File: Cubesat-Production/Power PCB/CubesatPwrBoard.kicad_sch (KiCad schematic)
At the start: 20 parts, among them J1 Conn_01x04_Female, J2 Conn_01x04_Female, J3 Conn_01x04_Female, J5 Conn_01x04_Female, J6 Conn_01x03_Female, J7 Conn_01x03_Female, J8 Conn_01x03_Female

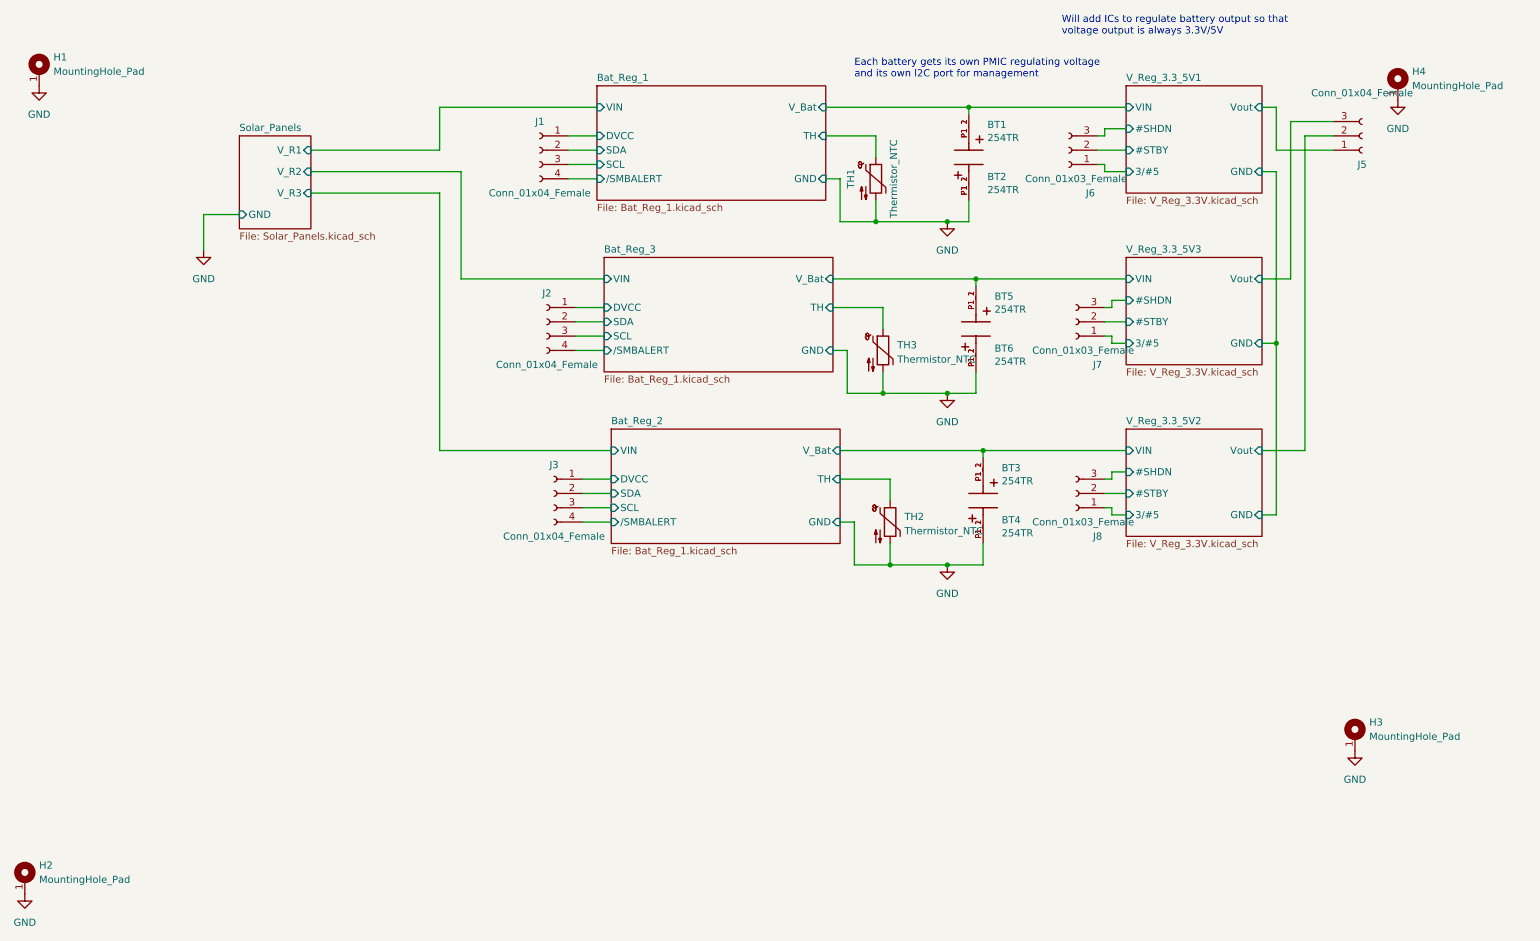
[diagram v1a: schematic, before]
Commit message: Small changes to board before moving to previous-revision
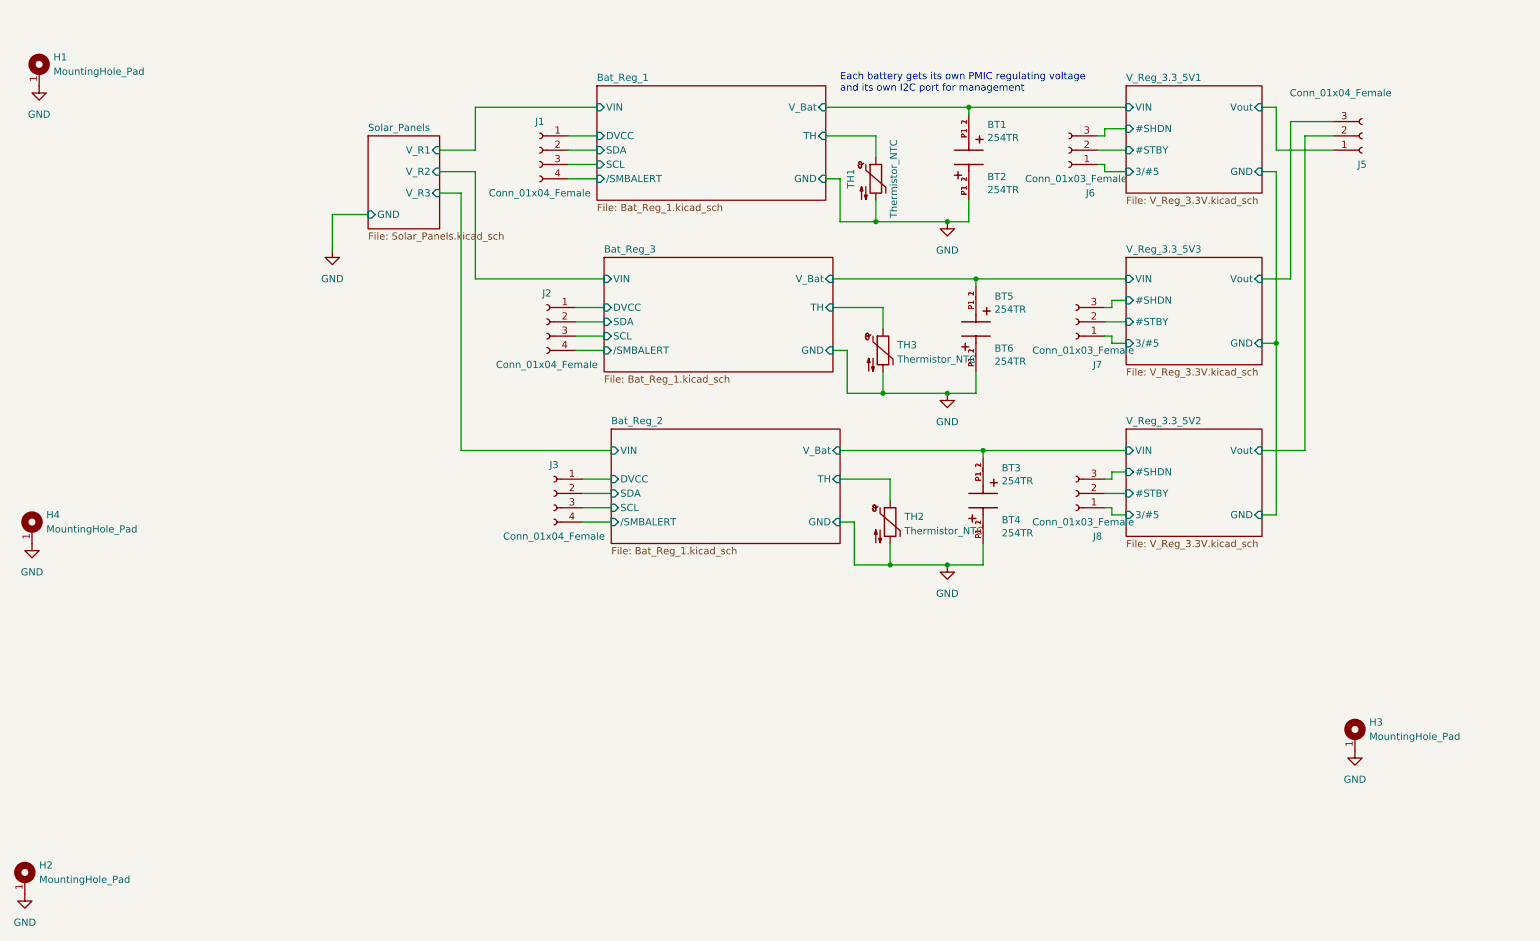
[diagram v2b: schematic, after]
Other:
- note removed: "Will add ICs to regulate battery output so that voltage output is always 3.3V/5V"
- moved on the sheet: H4
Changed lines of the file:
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@@
     (stroke (width 0) (type default) (color 0 0 0 0))
   )
-  (wire (pts (xy 60.96 55.88) (xy 67.31 55.88))
+  (wire (pts (xy 83.82 55.88) (xy 90.17 55.88))
     (stroke (width 0) (type default) (color 0 0 0 0))
   )
@@
     (stroke (width 0) (type default) (color 0 0 0 0))
   )
-  (wire (pts (xy 106.68 67.31) (xy 106.68 48.26))
+  (wire (pts (xy 109.22 67.31) (xy 109.22 48.26))
     (stroke (width 0) (type default) (color 0 0 0 0))
   )
@@
     (stroke (width 0) (type default) (color 0 0 0 0))
   )
-  (wire (pts (xy 80.01 44.45) (xy 102.87 44.45))
-    (stroke (width 0) (type default) (color 0 0 0 0))
-  )
   (wire (pts (xy 220.98 105.41) (xy 224.79 105.41))
     (stroke (width 0) (type default) (color 0 0 0 0))
   )
-  (wire (pts (xy 102.87 52.07) (xy 102.87 97.79))
+  (wire (pts (xy 106.68 52.07) (xy 106.68 97.79))
     (stroke (width 0) (type default) (color 0 0 0 0))
   )
@@
     (stroke (width 0) (type default) (color 0 0 0 0))
   )
-  (wire (pts (xy 102.87 97.79) (xy 133.35 97.79))
-    (stroke (width 0) (type default) (color 0 0 0 0))
-  )
   (wire (pts (xy 171.45 41.91) (xy 180.34 41.91))
     (stroke (width 0) (type default) (color 0 0 0 0))
@@
     (stroke (width 0) (type default) (color 0 0 0 0))
   )
+  (wire (pts (xy 102.87 52.07) (xy 106.68 52.07))
+    (stroke (width 0) (type default) (color 0 0 0 0))
+  )
   (wire (pts (xy 193.04 87.63) (xy 198.12 87.63))
     (stroke (width 0) (type default) (color 0 0 0 0))
@@
     (stroke (width 0) (type default) (color 0 0 0 0))
   )
-  (wire (pts (xy 60.96 62.23) (xy 60.96 55.88))
+  (wire (pts (xy 83.82 62.23) (xy 83.82 55.88))
+    (stroke (width 0) (type default) (color 0 0 0 0))
+  )
+  (wire (pts (xy 109.22 36.83) (xy 130.81 36.83))
     (stroke (width 0) (type default) (color 0 0 0 0))
   )
@@
     (stroke (width 0) (type default) (color 0 0 0 0))
   )
+  (wire (pts (xy 102.87 48.26) (xy 109.22 48.26))
+    (stroke (width 0) (type default) (color 0 0 0 0))
+  )
   (wire (pts (xy 222.25 109.22) (xy 224.79 109.22))
     (stroke (width 0) (type default) (color 0 0 0 0))
@@
     (stroke (width 0) (type default) (color 0 0 0 0))
   )
-  (wire (pts (xy 106.68 67.31) (xy 132.08 67.31))
-    (stroke (width 0) (type default) (color 0 0 0 0))
-  )
   (wire (pts (xy 172.72 67.31) (xy 198.12 67.31))
     (stroke (width 0) (type default) (color 0 0 0 0))
@@
     (stroke (width 0) (type default) (color 0 0 0 0))
   )
-  (wire (pts (xy 80.01 48.26) (xy 106.68 48.26))
-    (stroke (width 0) (type default) (color 0 0 0 0))
-  )
   (wire (pts (xy 173.99 97.79) (xy 199.39 97.79))
     (stroke (width 0) (type default) (color 0 0 0 0))
@@
     (stroke (width 0) (type default) (color 0 0 0 0))
   )
-  (wire (pts (xy 102.87 44.45) (xy 102.87 36.83))
+  (wire (pts (xy 109.22 44.45) (xy 109.22 36.83))
     (stroke (width 0) (type default) (color 0 0 0 0))
   )
@@
     (stroke (width 0) (type default) (color 0 0 0 0))
   )
+  (wire (pts (xy 102.87 44.45) (xy 109.22 44.45))
+    (stroke (width 0) (type default) (color 0 0 0 0))
+  )
   (wire (pts (xy 220.98 77.47) (xy 222.25 77.47))
     (stroke (width 0) (type default) (color 0 0 0 0))
   )
-  (wire (pts (xy 102.87 36.83) (xy 130.81 36.83))
-    (stroke (width 0) (type default) (color 0 0 0 0))
-  )
   (wire (pts (xy 180.34 57.15) (xy 193.04 57.15))
     (stroke (width 0) (type default) (color 0 0 0 0))
@@
     (stroke (width 0) (type default) (color 0 0 0 0))
   )
+  (wire (pts (xy 109.22 67.31) (xy 132.08 67.31))
+    (stroke (width 0) (type default) (color 0 0 0 0))
+  )
   (wire (pts (xy 176.53 118.11) (xy 182.88 118.11))
     (stroke (width 0) (type default) (color 0 0 0 0))
@@
     (stroke (width 0) (type default) (color 0 0 0 0))
   )
-  (wire (pts (xy 80.01 52.07) (xy 102.87 52.07))
+  (wire (pts (xy 106.68 97.79) (xy 133.35 97.79))
     (stroke (width 0) (type default) (color 0 0 0 0))
   )
@@
     (stroke (width 0) (type default) (color 0 0 0 0))
   )
-  (text "Will add ICs to regulate battery output so that\nvoltage output is always 3.3V/5V"
-    (at 213.36 24.13 0)
-    (effects (font (size 1.27 1.27)) (justify left bottom))
-  )
   (text "Each battery gets its own PMIC regulating voltage\nand its own I2C port for management"
-    (at 176.53 31.75 0)
+    (at 173.99 34.29 0)
     (effects (font (size 1.27 1.27)) (justify left bottom))
   )
@@
     (pin "3")
   )
-  (symbol (lib_id "power:GND") (at 273.05 35.56 0) (unit 1)
-    (in_bom yes) (on_board yes) (fields_autoplaced)
-    (property "Reference" "#PWR0115" (id 0) (at 273.05 41.91 0)
-      (effects (font (size 1.27 1.27)) hide)
-    )
-    (property "Value" "GND" (id 1) (at 273.05 40.64 0))
-    (property "Footprint" "" (id 2) (at 273.05 35.56 0)
-      (effects (font (size 1.27 1.27)) hide)
-    )
-    (property "Datasheet" "" (id 3) (at 273.05 35.56 0)
-      (effects (font (size 1.27 1.27)) hide)
-    )
-    (pin "1")
-  )
-  (symbol (lib_id "Mechanical:MountingHole_Pad") (at 273.05 33.02 0) (unit 1)
-    (in_bom yes) (on_board yes) (fields_autoplaced)
-    (property "Reference" "H4" (id 0) (at 275.59 30.4799 0)
-      (effects (font (size 1.27 1.27)) (justify left))
-    )
-    (property "Value" "MountingHole_Pad" (id 1) (at 275.59 33.0199 0)
-      (effects (font (size 1.27 1.27)) (justify left))
-    )
-    (property "Footprint" "MountingHole:MountingHole_4.3mm_M4_DIN965_Pad" (id 2) (at 273.05 33.02 0)
-      (effects (font (size 1.27 1.27)) hide)
-    )
-    (property "Datasheet" "~" (id 3) (at 273.05 33.02 0)
+  (symbol (lib_id "power:GND") (at 30.48 114.3 0) (unit 1)
+    (in_bom yes) (on_board yes) (fields_autoplaced)
+    (property "Reference" "#PWR0115" (id 0) (at 30.48 120.65 0)
+      (effects (font (size 1.27 1.27)) hide)
+    )
+    (property "Value" "GND" (id 1) (at 30.48 119.38 0))
+    (property "Footprint" "" (id 2) (at 30.48 114.3 0)
+      (effects (font (size 1.27 1.27)) hide)
+    )
+    (property "Datasheet" "" (id 3) (at 30.48 114.3 0)
+      (effects (font (size 1.27 1.27)) hide)
+    )
+    (pin "1")
+  )
+  (symbol (lib_id "Mechanical:MountingHole_Pad") (at 30.48 111.76 0) (unit 1)
+    (in_bom yes) (on_board yes) (fields_autoplaced)
+    (property "Reference" "H4" (id 0) (at 33.02 109.2199 0)
+      (effects (font (size 1.27 1.27)) (justify left))
+    )
+    (property "Value" "MountingHole_Pad" (id 1) (at 33.02 111.7599 0)
+      (effects (font (size 1.27 1.27)) (justify left))
+    )
+    (property "Footprint" "MountingHole:MountingHole_4.3mm_M4_DIN965_Pad" (id 2) (at 30.48 111.76 0)
+      (effects (font (size 1.27 1.27)) hide)
+    )
+    (property "Datasheet" "~" (id 3) (at 30.48 111.76 0)
       (effects (font (size 1.27 1.27)) hide)
     )
@@
     (in_bom yes) (on_board yes)
     (property "Reference" "J5" (id 0) (at 266.7 46.99 0))
-    (property "Value" "Conn_01x04_Female" (id 1) (at 266.7 34.29 0))
+    (property "Value" "Conn_01x04_Female" (id 1) (at 262.89 34.29 0))
     (property "Footprint" "Connector_PinSocket_2.54mm:PinSocket_1x03_P2.54mm_Vertical" (id 2) (at 266.7 41.91 0)
       (effects (font (size 1.27 1.27)) hide)
@@
     (pin "3")
   )
-  (symbol (lib_id "power:GND") (at 60.96 62.23 0) (unit 1)
-    (in_bom yes) (on_board yes) (fields_autoplaced)
-    (property "Reference" "#PWR0101" (id 0) (at 60.96 68.58 0)
-      (effects (font (size 1.27 1.27)) hide)
-    )
-    (property "Value" "GND" (id 1) (at 60.96 67.31 0))
-    (property "Footprint" "" (id 2) (at 60.96 62.23 0)
-      (effects (font (size 1.27 1.27)) hide)
-    )
-    (property "Datasheet" "" (id 3) (at 60.96 62.23 0)
+  (symbol (lib_id "power:GND") (at 83.82 62.23 0) (unit 1)
+    (in_bom yes) (on_board yes) (fields_autoplaced)
+    (property "Reference" "#PWR0101" (id 0) (at 83.82 68.58 0)
+      (effects (font (size 1.27 1.27)) hide)
+    )
+    (property "Value" "GND" (id 1) (at 83.82 67.31 0))
+    (property "Footprint" "" (id 2) (at 83.82 62.23 0)
+      (effects (font (size 1.27 1.27)) hide)
+    )
+    (property "Datasheet" "" (id 3) (at 83.82 62.23 0)
       (effects (font (size 1.27 1.27)) hide)
     )
@@
     )
   )
-  (sheet (at 67.31 41.91) (size 12.7 16.51) (fields_autoplaced)
+  (sheet (at 90.17 41.91) (size 12.7 16.51) (fields_autoplaced)
     (stroke (width 0.1524) (type solid) (color 0 0 0 0))
     (fill (color 0 0 0 0.0000))
-    (property "Sheet name" "Solar_Panels" (id 0) (at 67.31 41.1984 0)
+    (property "Sheet name" "Solar_Panels" (id 0) (at 90.17 41.1984 0)
       (effects (font (size 1.27 1.27)) (justify left bottom))
     )
-    (property "Sheet file" "Solar_Panels.kicad_sch" (id 1) (at 67.31 59.0046 0)
+    (property "Sheet file" "Solar_Panels.kicad_sch" (id 1) (at 90.17 59.0046 0)
       (effects (font (size 1.27 1.27)) (justify left top))
     )
-    (pin "GND" input (at 67.31 55.88 180)
-      (effects (font (size 1.27 1.27)) (justify left))
-    )
-    (pin "V_R3" input (at 80.01 52.07 0)
-      (effects (font (size 1.27 1.27)) (justify right))
-    )
-    (pin "V_R2" input (at 80.01 48.26 0)
-      (effects (font (size 1.27 1.27)) (justify right))
-    )
-    (pin "V_R1" input (at 80.01 44.45 0)
-      (effects (font (size 1.27 1.27)) (justify right))
-    )
+    (pin "GND" input (at 90.17 55.88 180)
+      (effects (font (size 1.27 1.27)) (justify left))
+    )
+    (pin "V_R3" input (at 102.87 52.07 0)
+      (effects (font (size 1.27 1.27)) (justify right))
+    )
+    (pin "V_R2" input (at 102.87 48.26 0)
+      (effects (font (size 1.27 1.27)) (justify right))
+    )
+    (pin "V_R1" input (at 102.87 44.45 0)
+      (effects (font (size 1.27 1.27)) (justify right))
+    )
